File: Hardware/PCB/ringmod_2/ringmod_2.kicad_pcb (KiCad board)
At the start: 2 copper layers, 1 part

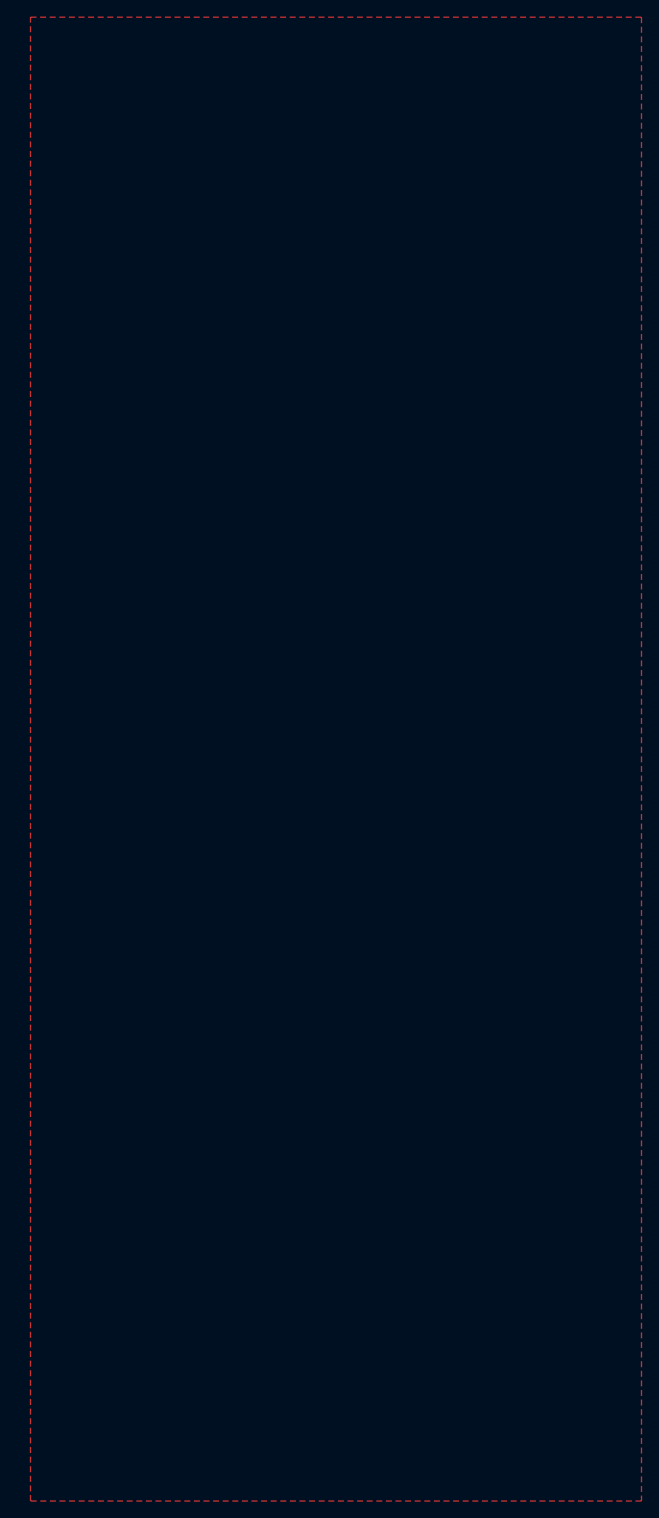
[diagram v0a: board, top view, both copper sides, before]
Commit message: rm first design; add new holes image
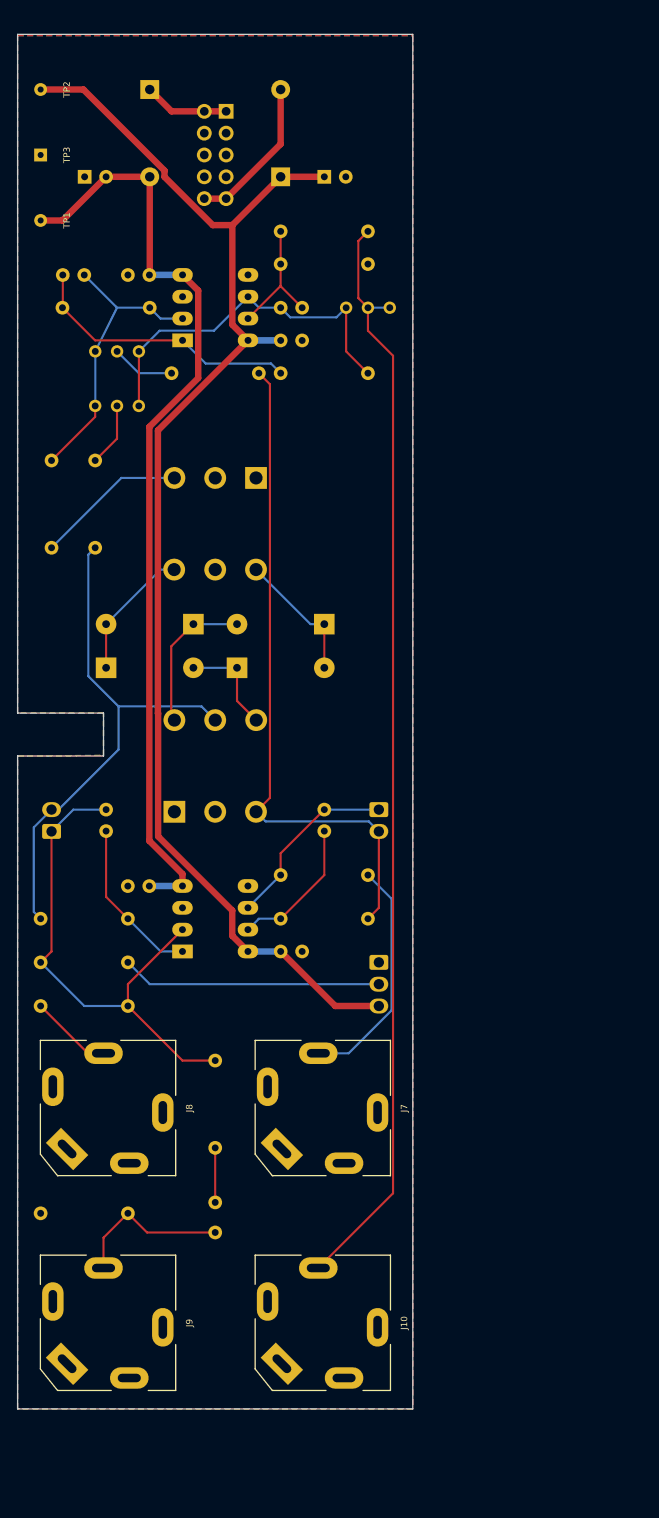
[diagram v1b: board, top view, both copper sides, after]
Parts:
- added C1: 47pF, ao_tht:C_Disc_D3.0mm_W1.6mm_P2.50mm, B.Cu at (112.7, 115.2)
- added C10: 100nF, ao_tht:C_Disc_D3.0mm_W1.6mm_P2.50mm, B.Cu at (89.8, 124.1)
- added C11: 100nF, ao_tht:C_Disc_D3.0mm_W1.6mm_P2.50mm, B.Cu at (89.8, 53.0)
- added C2: 47pF, ao_tht:C_Disc_D3.0mm_W1.6mm_P2.50mm, B.Cu at (84.8, 53.0)
- added C3: 10uF, ao_tht:C_Radial_D8.0mm_H11.5mm_P3.50mm, B.Cu at (100.0, 161.0)
- added C4: 47pF, ao_tht:C_Disc_D3.0mm_W1.6mm_P2.50mm, B.Cu at (87.3, 115.2)
- added C5: 47pF, ao_tht:C_Disc_D3.0mm_W1.6mm_P2.50mm, B.Cu at (107.6, 56.8)
- added C6: 10uF, ao_tht:CP_Radial_D6.3mm_P2.50mm, B.Cu at (112.7, 41.6)
- added C7: 100nF, ao_tht:C_Disc_D3.0mm_W1.6mm_P2.50mm, B.Cu at (107.6, 131.8)
- added C8: 100nF, ao_tht:C_Disc_D3.0mm_W1.6mm_P2.50mm, B.Cu at (107.6, 60.6)
- added C9: 10uF, ao_tht:CP_Radial_D6.3mm_P2.50mm, B.Cu at (84.8, 41.6)
- added D1: 1N695, ringmod:D_DO-7_P10.16mm_Horizontal, B.Cu at (87.3, 98.7)
- added D2: 1N695, ringmod:D_DO-7_P10.16mm_Horizontal, B.Cu at (97.5, 93.7)
- added D3: 1N695, ringmod:D_DO-7_P10.16mm_Horizontal, B.Cu at (102.5, 98.7)
- added D4: 1N695, ringmod:D_DO-7_P10.16mm_Horizontal, B.Cu at (112.7, 93.7)
- added D5: 1N5817, ao_tht:D_DO-41_SOD81_P10.16mm_Horizontal, B.Cu at (107.6, 41.6)
- added D6: 1N5817, ao_tht:D_DO-41_SOD81_P10.16mm_Horizontal, B.Cu at (92.4, 31.4)
- added J1: 3_pin_Molex_header, ao_tht:Molex_KK-254_AE-6410-03A_1x03_P2.54mm_Vertical, B.Cu at (119.0, 133.0)
- added J10: AudioJack2, ao_tht:Jack_6.35mm_PJ_629HAN_slots, F.Cu at (112.5, 175.0)
- added J11: Synth_power_2x5, ao_tht:Power_Header, B.Cu at (101.3, 34.0)
- added J3: 2_pin_Molex_header, ao_tht:Molex_KK-254_AE-6410-02A_1x02_P2.54mm_Vertical, B.Cu at (81.0, 117.8)
- added J5: 2_pin_Molex_header, ao_tht:Molex_KK-254_AE-6410-02A_1x02_P2.54mm_Vertical, B.Cu at (119.0, 115.2)
- added J7: AudioJack2, ao_tht:Jack_6.35mm_PJ_629HAN_slots, F.Cu at (112.5, 150.0)
- added J8: AudioJack2, ao_tht:Jack_6.35mm_PJ_629HAN_slots, F.Cu at (87.5, 150.0)
- added J9: AudioJack2, ao_tht:Jack_6.35mm_PJ_629HAN_slots, F.Cu at (87.5, 175.0)
- added R1: 100k, ao_tht:R_Axial_DIN0207_L6.3mm_D2.5mm_P10.16mm_Horizontal, B.Cu at (117.8, 122.9)
- added R10: 330R, ao_tht:R_Axial_DIN0207_L6.3mm_D2.5mm_P10.16mm_Horizontal, B.Cu at (89.8, 127.9)
- added R11: 100k, ao_tht:R_Axial_DIN0207_L6.3mm_D2.5mm_P10.16mm_Horizontal, B.Cu at (86.0, 84.8)
- added R12: 33k, ao_tht:R_Axial_DIN0207_L6.3mm_D2.5mm_P10.16mm_Horizontal, B.Cu at (107.6, 64.4)
- added R13: 1k, ao_tht:R_Axial_DIN0207_L6.3mm_D2.5mm_P10.16mm_Horizontal, B.Cu at (107.6, 47.9)
- added R14: 100k, ao_tht:R_Axial_DIN0207_L6.3mm_D2.5mm_P10.16mm_Horizontal, B.Cu at (117.8, 51.7)
- added R2: 330R, ao_tht:R_Axial_DIN0207_L6.3mm_D2.5mm_P10.16mm_Horizontal, B.Cu at (107.6, 127.9)
- added R3: 100k, ao_tht:R_Axial_DIN0207_L6.3mm_D2.5mm_P10.16mm_Horizontal, B.Cu at (105.1, 64.4)
- added R4: 100k, ao_tht:R_Axial_DIN0207_L6.3mm_D2.5mm_P10.16mm_Horizontal, B.Cu at (79.7, 138.1)
- added R5: 100k, ao_tht:R_Axial_DIN0207_L6.3mm_D2.5mm_P10.16mm_Horizontal, B.Cu at (92.4, 56.8)
- added R6: 100k, ao_tht:R_Axial_DIN0207_L6.3mm_D2.5mm_P10.16mm_Horizontal, B.Cu at (81.0, 84.8)
- added R7: 100k, ao_tht:R_Axial_DIN0207_L6.3mm_D2.5mm_P10.16mm_Horizontal, B.Cu at (100.0, 154.6)
- added R8: 1M, ao_tht:R_Axial_DIN0207_L6.3mm_D2.5mm_P10.16mm_Horizontal, B.Cu at (89.8, 162.2)
- added R9: 330R, ao_tht:R_Axial_DIN0207_L6.3mm_D2.5mm_P10.16mm_Horizontal, B.Cu at (89.8, 133.0)
- added RV7: 20k, ao_tht:Potentiometer_Bourns_3296W_Vertical_standard, B.Cu at (91.1, 68.2)
- added RV8: 20k, ao_tht:Potentiometer_Bourns_3296W_Vertical_standard, B.Cu at (91.1, 61.9)
- added RV9: 100k, ao_tht:Potentiometer_Bourns_3296W_Vertical_standard, B.Cu at (115.2, 56.8)
- added TP1: -12V, ao_tht:TestPoint_THTPad_D1.5mm_Drill0.7mm, B.Cu at (79.7, 46.7)
- added TP2: +12V, ao_tht:TestPoint_THTPad_D1.5mm_Drill0.7mm, B.Cu at (79.7, 31.4)
- added TP3: GND, ao_tht:TestPoint_THTPad_1.5x1.5mm_Drill0.7mm, B.Cu at (79.7, 39.0)
- added TR1: TY-141P, ringmod:Transformer_TY-141P, B.Cu at (95.2, 115.5)
- added TR2: TY-141P, ringmod:Transformer_TY-141P, B.Cu at (104.7, 76.6)
- added U1: NE5532, ao_tht:DIP-8_W7.62mm_Socket_LongPads, B.Cu at (96.2, 131.8)
- added U2: TL072, ao_tht:DIP-8_W7.62mm_Socket_LongPads, B.Cu at (96.2, 60.6)
- GRAF1: footprint ringmod_panel:ringmod_panel_2_holes -> ringmod:ringmod_panel_2_holes
- moved GRAF1 14.1 mm to (100.0, 100.0)
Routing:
- net +12V: track 0.00 -> 158.0 mm
- net /Main PCB/OUT: track 0.00 -> 129.0 mm
- net -12V: track 0.00 -> 109.8 mm
- net /Main PCB/SIGLVL_CW: track 0.00 -> 78.2 mm
- net /Main PCB/CARRLVL_CW: track 0.00 -> 61.8 mm
- net /Main PCB/CARRLVL_CCW: track 0.00 -> 59.7 mm
- net Net-(C5-Pad1): track 0.00 -> 43.2 mm
- net Net-(C2-Pad1): track 0.00 -> 34.0 mm
- net Net-(C2-Pad2): track 0.00 -> 32.4 mm
- net /Main PCB/UNBAL_WIP: track 0.00 -> 30.3 mm
- net /Main PCB/SIG IN: track 0.00 -> 27.5 mm
- net /Main PCB/SIGLVL_CCW: track 0.00 -> 21.5 mm
- net Net-(C4-Pad2): track 0.00 -> 19.2 mm
- net /Main PCB/AC CARR IN: track 0.00 -> 18.6 mm
- net /Main PCB/+12_IN: track 0.00 -> 17.9 mm
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- added copper zone on B.Cu, net GND
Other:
- board outline added: 46 x 160 mm
